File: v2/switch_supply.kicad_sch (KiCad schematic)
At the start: 9 parts, among them U11 ADG419BN, U12 ADG419BN, U7 ADG419BN

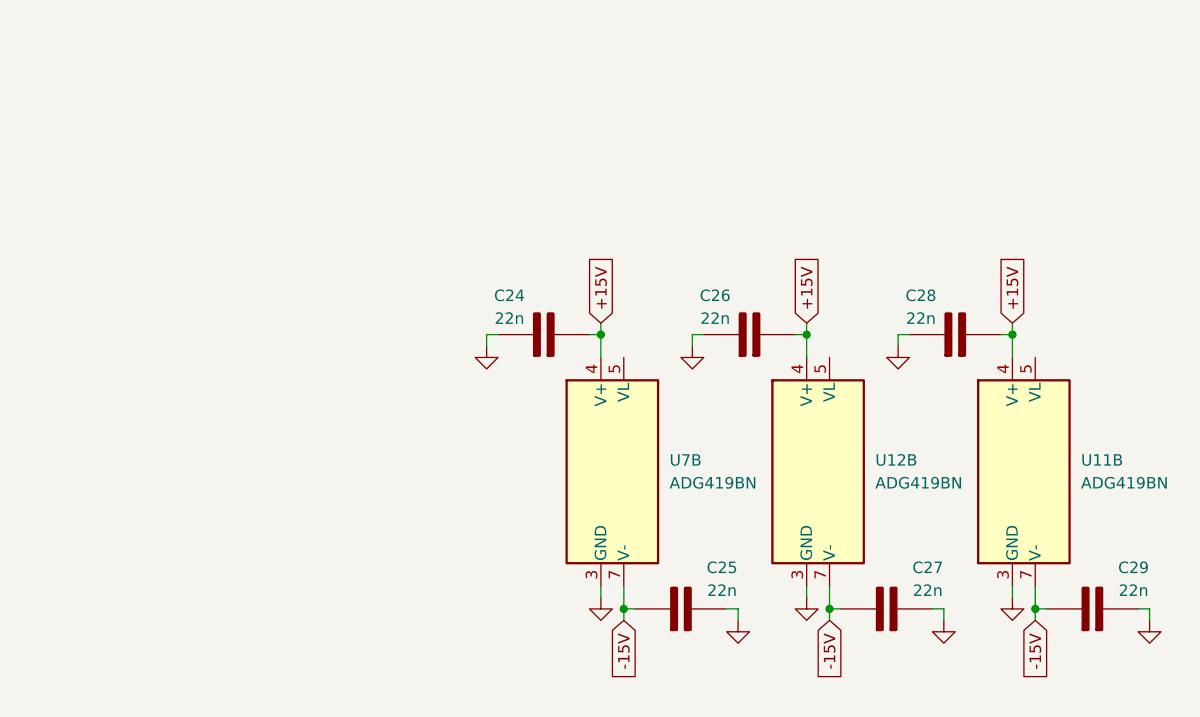
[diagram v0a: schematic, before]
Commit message: Almostt finished everything, just finishing details
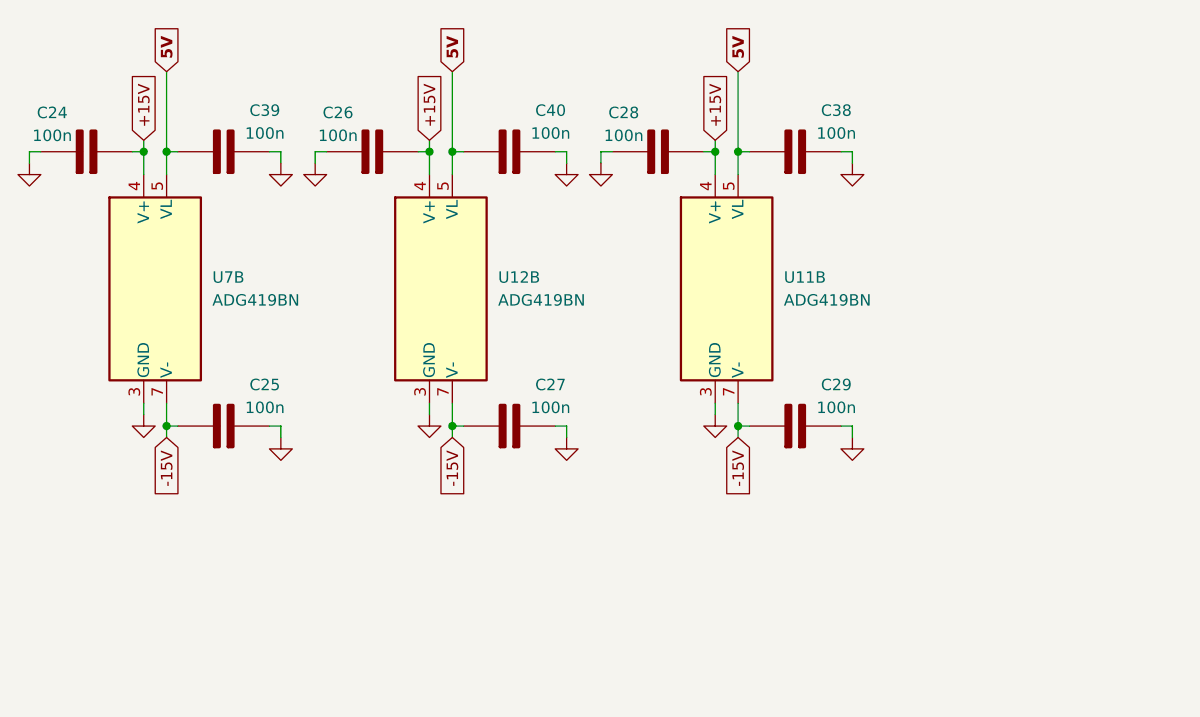
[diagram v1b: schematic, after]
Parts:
- added C38, C39, C40: 100n, symbol custom:C_Basic
- C24, C25, C26, C27, C28, C29: value 22n -> 100n
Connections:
- net GND: now also C38., C39., C40.
- net 5V: now reaches U7.5 (VL)
- net 5V: now also U11.5 (VL), U12.5 (VL), C38., C39., C40.
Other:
- moved on the sheet: C24, C25, C26, C27, C28, C29, U11B, U12B, U7B

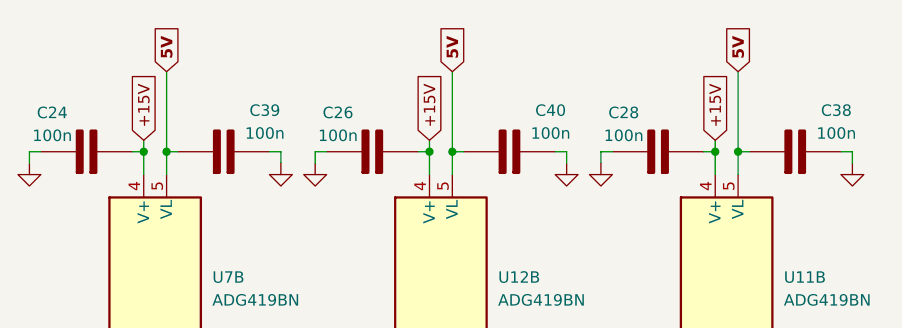
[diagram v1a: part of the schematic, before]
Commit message: Almost finished v2
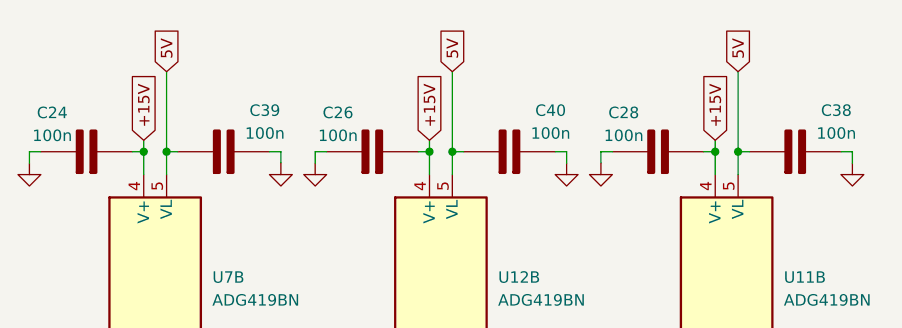
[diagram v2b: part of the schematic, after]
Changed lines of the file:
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@@
 			(font
 				(size 1.27 1.27)
-				(thickness 0.254)
-				(bold yes)
+				(thickness 0.1588)
 			)
 			(justify left)
 		)
 		(property "Intersheetrefs" "${INTERSHEET_REFS}"
-			(at 82.55 39.9607 90)
+			(at 82.55 40.4367 90)
 			(hide yes)
 			(show_name no)
@@
 			(font
 				(size 1.27 1.27)
-				(thickness 0.254)
-				(bold yes)
+				(thickness 0.1588)
 			)
 			(justify left)
 		)
 		(property "Intersheetrefs" "${INTERSHEET_REFS}"
-			(at 114.3 39.9607 90)
+			(at 114.3 40.4367 90)
 			(hide yes)
 			(show_name no)
@@
 			(font
 				(size 1.27 1.27)
-				(thickness 0.254)
-				(bold yes)
+				(thickness 0.1588)
 			)
 			(justify left)
 		)
 		(property "Intersheetrefs" "${INTERSHEET_REFS}"
-			(at 146.05 39.9607 90)
+			(at 146.05 40.4367 90)
 			(hide yes)
 			(show_name no)
